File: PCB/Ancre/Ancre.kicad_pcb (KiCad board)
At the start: 2 copper layers, 72.2 x 60.7 mm, 18 parts, among them IC1 TCAN1051VDRQ1, U1 OKI-78SR-5_1.5-W36-C, U2 DB301V-5.0-2P, U3 DB301V-5.0-2P, U6 DB301V-5.0-2P, U7 DB301V-5.0-2P

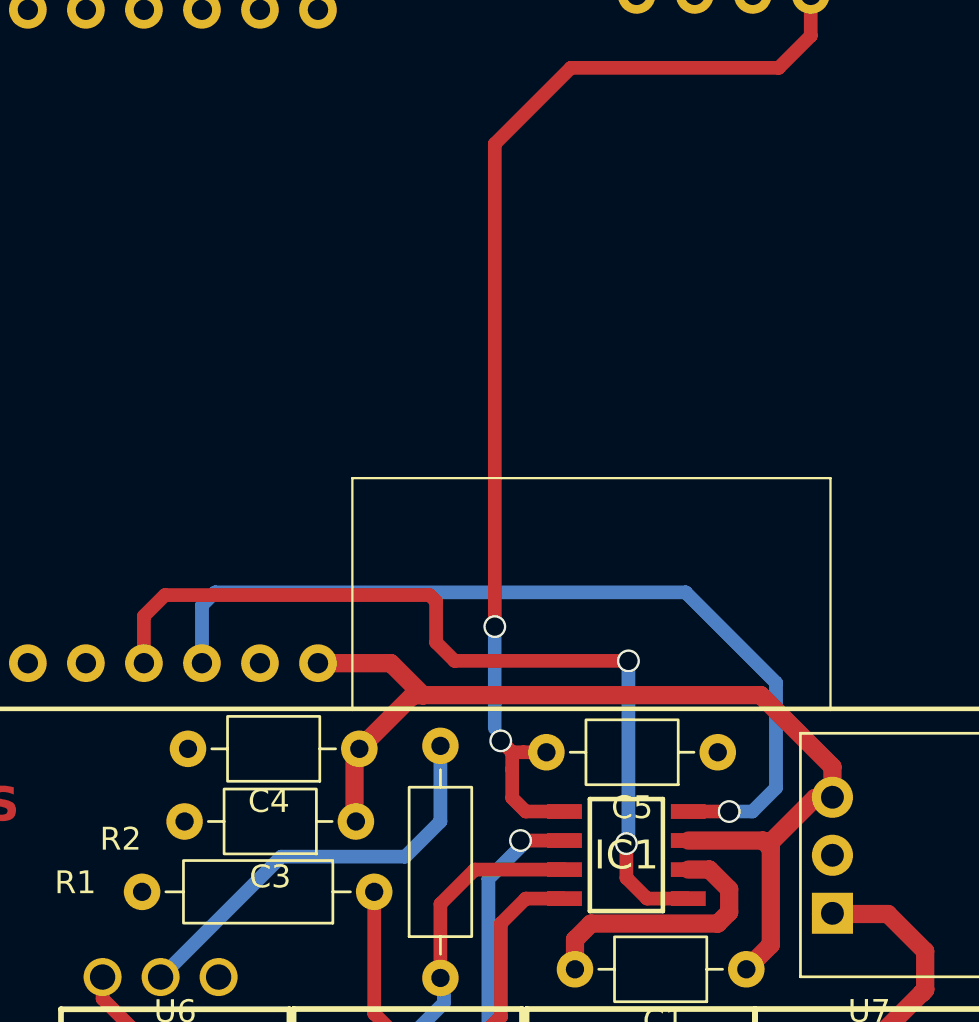
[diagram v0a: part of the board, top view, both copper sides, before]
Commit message: gbr
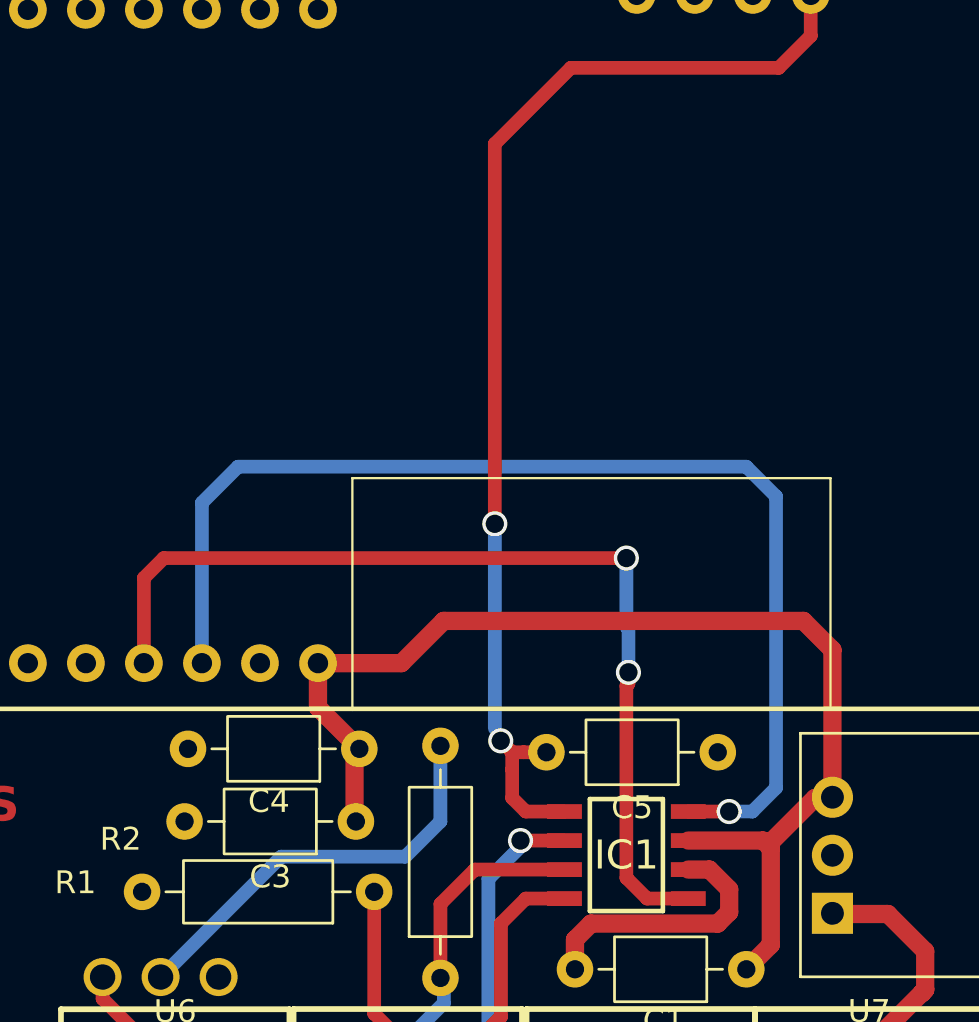
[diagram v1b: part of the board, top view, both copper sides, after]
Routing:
- net Net-(IC1-RXD): track 38.4 -> 50.4 mm
- net +5V: track 46.3 -> 51.5 mm
- net Net-(IC1-TXD): track 38.5 -> 42.4 mm
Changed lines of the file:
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@@
 		(filling no)
 		(pcbplotparams
-			(layerselection 0x00000000_00000000_55555555_5755f5ff)
-			(plot_on_all_layers_selection 0x00000000_00000000_00000000_00000000)
+			(layerselection 0x00000000_00000000_55555555_57555555)
+			(plot_on_all_layers_selection 0x00000000_00000000_00000000_02000000)
 			(disableapertmacros no)
 			(usegerberextensions no)
@@
 			(outputformat 1)
 			(mirror no)
-			(drillshape 1)
+			(drillshape 0)
 			(scaleselection 1)
 			(outputdirectory "")
@@
 	(via
 		(at 244.365 83.865)
-		(size 1)
+		(size 1.1)
 		(drill 0.8)
 		(layers "F.Cu" "B.Cu")
@@
 	)
 	(segment
+		(start 256.75 74.25)
+		(end 258.02 75.52)
+		(width 0.8)
+		(layer "F.Cu")
+		(net "+5V")
+	)
+	(segment
 		(start 255.32 83.94)
 		(end 255.32 84.2)
@@
 	)
 	(segment
-		(start 240.1 77.51)
-		(end 240.11 77.5)
-		(width 0.8)
-		(layer "F.Cu")
-		(net "+5V")
-	)
-	(segment
-		(start 254.88 77.5)
-		(end 258.02 80.64)
-		(width 0.8)
-		(layer "F.Cu")
-		(net "+5V")
-	)
-	(segment
-		(start 238.69 76.1)
-		(end 235.5 76.1)
+		(start 239.15 76.1)
+		(end 241 74.25)
 		(width 0.8)
 		(layer "F.Cu")
@@
 	)
 	(segment
-		(start 240.1 77.51)
-		(end 238.69 76.1)
+		(start 258.02 75.52)
+		(end 258.02 81.97)
 		(width 0.8)
 		(layer "F.Cu")
@@
 	)
 	(segment
-		(start 239.65 77.51)
-		(end 237.31 79.85)
+		(start 258.02 81.97)
+		(end 257.99 82)
 		(width 0.8)
 		(layer "F.Cu")
@@
 	)
 	(segment
-		(start 258.02 81.97)
-		(end 257.99 82)
+		(start 241 74.25)
+		(end 256.75 74.25)
 		(width 0.8)
 		(layer "F.Cu")
@@
 	)
 	(segment
-		(start 258.02 80.64)
-		(end 258.02 81.97)
+		(start 235.5 78.04)
+		(end 237.31 79.85)
 		(width 0.8)
 		(layer "F.Cu")
@@
 	)
 	(segment
-		(start 240.11 77.5)
-		(end 254.88 77.5)
+		(start 235.5 76.1)
+		(end 235.5 78.04)
 		(width 0.8)
 		(layer "F.Cu")
@@
 	)
 	(segment
-		(start 240.1 77.51)
-		(end 239.65 77.51)
+		(start 235.5 76.1)
+		(end 239.15 76.1)
 		(width 0.8)
 		(layer "F.Cu")
@@
 	)
 	(segment
-		(start 240.67 75.19)
-		(end 240.67 73.4)
+		(start 228.75 71.5)
+		(end 227.88 72.37)
 		(width 0.6)
 		(layer "F.Cu")
@@
 	)
 	(segment
-		(start 249.905 86.405)
-		(end 251.711 86.405)
-		(width 0.6)
-		(layer "F.Cu")
-		(net "Net-(IC1-TXD)")
-	)
-	(segment
-		(start 240.67 73.4)
-		(end 240.39 73.12)
+		(start 249.09 77)
+		(end 249 77.09)
 		(width 0.6)
 		(layer "F.Cu")
@@
 	)
 	(segment
-		(start 227.88 74.04)
-		(end 227.88 76.1)
-		(width 0.6)
-		(layer "F.Cu")
-		(net "Net-(IC1-TXD)")
-	)
-	(segment
-		(start 228.8 73.12)
-		(end 227.88 74.04)
+		(start 249.09 76.5)
+		(end 249.09 77)
 		(width 0.6)
 		(layer "F.Cu")
@@
 	)
 	(segment
-		(start 240.39 73.12)
-		(end 228.8 73.12)
+		(start 249 77.09)
+		(end 249 85.5)
 		(width 0.6)
 		(layer "F.Cu")
@@
 	)
 	(segment
-		(start 241.48 76)
-		(end 240.67 75.19)
+		(start 249 71.5)
+		(end 228.75 71.5)
 		(width 0.6)
 		(layer "F.Cu")
@@
 	)
 	(segment
-		(start 249.09 76)
-		(end 241.48 76)
+		(start 227.88 72.37)
+		(end 227.88 76.1)
 		(width 0.6)
 		(layer "F.Cu")
@@
 	)
 	(segment
-		(start 249 84)
-		(end 249 85.5)
+		(start 249.905 86.405)
+		(end 251.711 86.405)
 		(width 0.6)
 		(layer "F.Cu")
@@
 	)
 	(via
-		(at 249.09 76)
-		(size 1)
+		(at 249 71.5)
+		(size 1.1)
 		(drill 0.8)
 		(layers "F.Cu" "B.Cu")
@@
 	)
 	(via
-		(at 249 84)
-		(size 1)
+		(at 249.09 76.5)
+		(size 1.1)
 		(drill 0.8)
 		(layers "F.Cu" "B.Cu")
@@
 	)
 	(segment
-		(start 249.09 76)
-		(end 249.09 83.91)
+		(start 249 71.5)
+		(end 249 74.5)
 		(width 0.6)
 		(layer "B.Cu")
@@
 	)
 	(segment
-		(start 249.09 83.91)
-		(end 249 84)
+		(start 249 74.5)
+		(end 249.09 74.59)
+		(width 0.6)
+		(layer "B.Cu")
+		(net "Net-(IC1-TXD)")
+	)
+	(segment
+		(start 249.09 74.59)
+		(end 249.09 76.5)
 		(width 0.6)
 		(layer "B.Cu")
@@
 	(via
 		(at 253.5 82.595)
-		(size 1)
+		(size 1.1)
 		(drill 0.8)
 		(layers "F.Cu" "B.Cu")
@@
 	)
 	(segment
-		(start 255.55 81.56)
-		(end 255.55 76.955)
+		(start 255.55 68.8)
+		(end 254.25 67.5)
 		(width 0.6)
 		(layer "B.Cu")
@@
 	)
 	(segment
-		(start 251.595 73)
-		(end 231 73)
+		(start 254.25 67.5)
+		(end 232 67.5)
 		(width 0.6)
 		(layer "B.Cu")
@@
 	)
 	(segment
-		(start 254.515 82.595)
-		(end 255.55 81.56)
+		(start 232 67.5)
+		(end 230.42 69.08)
 		(width 0.6)
 		(layer "B.Cu")
@@
 	)
 	(segment
-		(start 255.55 76.955)
-		(end 251.595 73)
+		(start 253.5 82.595)
+		(end 254.515 82.595)
 		(width 0.6)
 		(layer "B.Cu")
@@
 	)
 	(segment
-		(start 231 73)
-		(end 230.42 73.58)
+		(start 254.515 82.595)
+		(end 255.55 81.56)
 		(width 0.6)
 		(layer "B.Cu")
@@
 	)
 	(segment
-		(start 230.42 73.58)
+		(start 230.42 69.08)
 		(end 230.42 76.1)
 		(width 0.6)
@@
 	)
 	(segment
-		(start 253.5 82.595)
-		(end 254.515 82.595)
+		(start 255.55 81.56)
+		(end 255.55 68.8)
 		(width 0.6)
 		(layer "B.Cu")
@@
 	)
 	(segment
-		(start 243.24 53.37)
-		(end 246.57 50.04)
+		(start 257.0708 48.6392)
+		(end 257.0708 46.8462)
 		(width 0.6)
 		(layer "F.Cu")
@@
 	)
 	(segment
-		(start 244 82)
-		(end 244.595 82.595)
+		(start 243.24 53.37)
+		(end 246.57 50.04)
 		(width 0.6)
 		(layer "F.Cu")
@@
 	)
 	(segment
-		(start 243.24 74.5)
-		(end 243.24 53.37)
+		(start 246.57 50.04)
+		(end 255.67 50.04)
 		(width 0.6)
 		(layer "F.Cu")
@@
 	)
 	(segment
-		(start 244 80)
-		(end 243.5 79.5)
+		(start 244 82)
+		(end 244.595 82.595)
 		(width 0.6)
 		(layer "F.Cu")
@@
 	)
 	(segment
-		(start 255.67 50.04)
-		(end 257.0708 48.6392)
+		(start 244 80)
+		(end 243.5 79.5)
 		(width 0.6)
 		(layer "F.Cu")
@@
 	)
 	(segment
-		(start 246.57 50.04)
-		(end 255.67 50.04)
+		(start 255.67 50.04)
+		(end 257.0708 48.6392)
 		(width 0.6)
 		(layer "F.Cu")
@@
 	)
 	(segment
-		(start 257.0708 48.6392)
-		(end 257.0708 46.8462)
+		(start 243.24 70)
+		(end 243.24 53.37)
 		(width 0.6)
 		(layer "F.Cu")
@@
 	(via
 		(at 243.5 79.5)
-		(size 1)
+		(size 1.1)
 		(drill 0.8)
 		(layers "F.Cu" "B.Cu")
@@
 	)
 	(via
-		(at 243.24 74.5)
-		(size 1)
+		(at 243.24 70)
+		(size 1.1)
 		(drill 0.8)
 		(layers "F.Cu" "B.Cu")
@@
 	)
 	(segment
-		(start 243.24 78.95)
-		(end 243.24 74.5)
-		(width 0.6)
-		(layer "B.Cu")
-		(net "Net-(IC1-NC)")
-	)
-	(segment
 		(start 243.5 79.5)
 		(end 243.5 79.21)
@@
 		(layer "B.Cu")
 		(net "Net-(IC1-NC)")
+	)
+	(segment
+		(start 243.24 78.95)
+		(end 243.24 70)
+		(width 0.6)
+		(layer "B.Cu")
+		(net "Net-(IC1-NC)")
